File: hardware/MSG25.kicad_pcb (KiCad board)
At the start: 2 copper layers, 48 parts, among them J101 USART, J102 STLink, U105 AMS1117-5, U106 AMS1117-3.3, U202 STM32L431RCTx, U501 MCP2561-E-SN

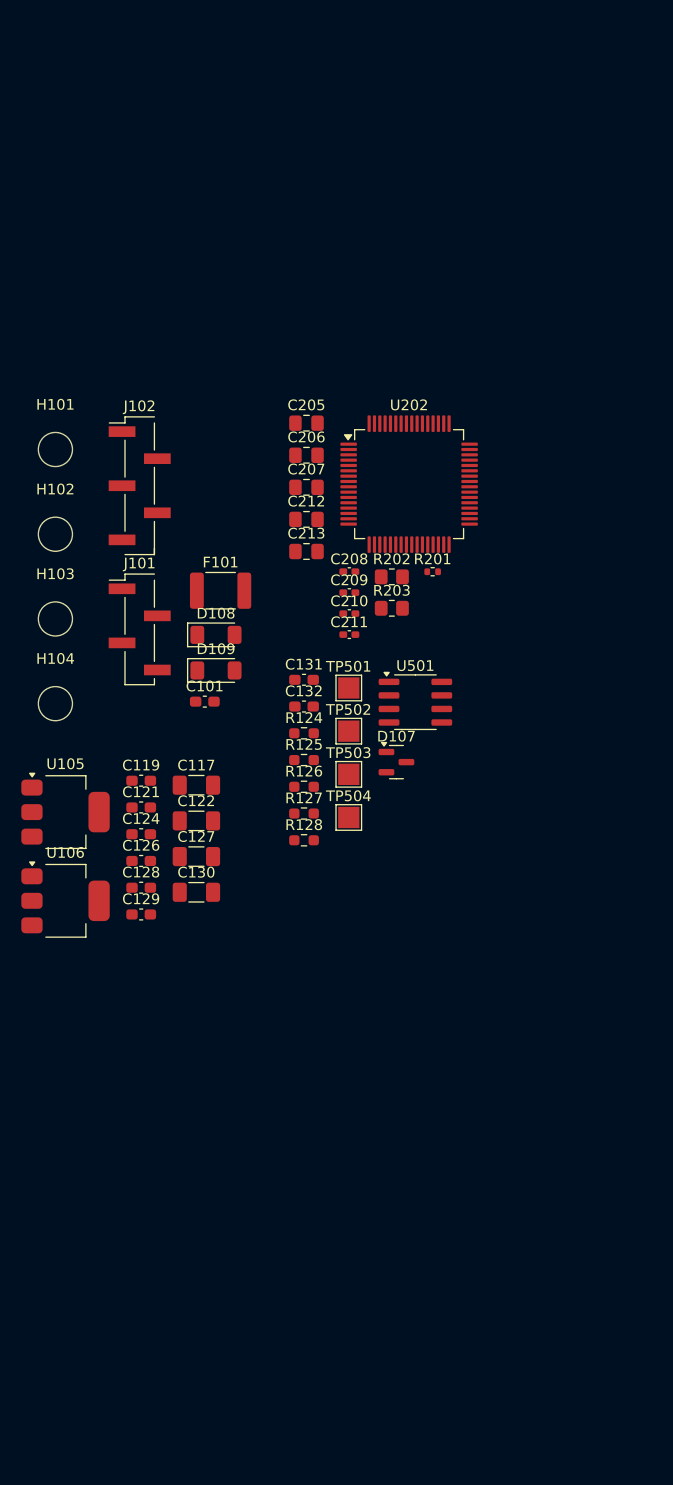
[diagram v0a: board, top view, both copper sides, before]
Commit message: Placa Finalizada para revisão
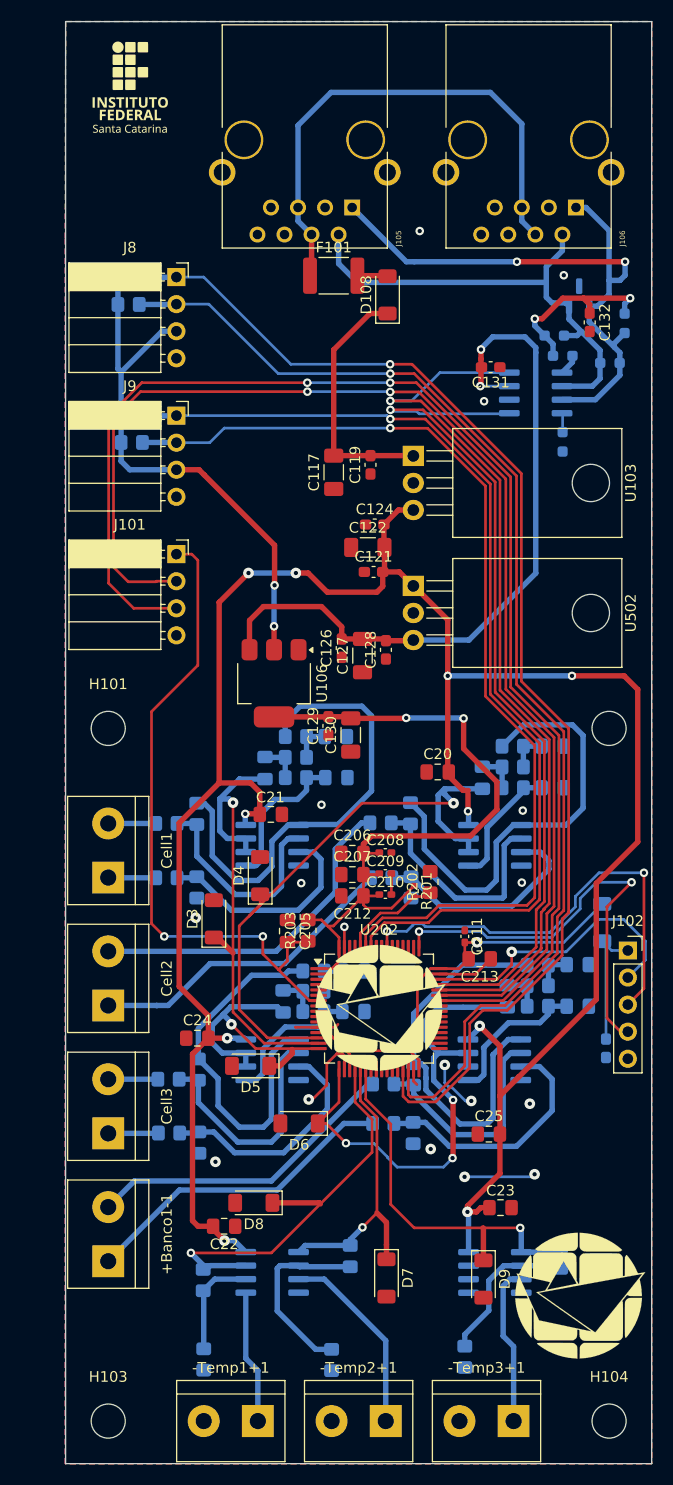
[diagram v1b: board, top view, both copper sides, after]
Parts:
- removed TP501: TxCAN, TestPoint:TestPoint_Pad_2.0x2.0mm
- removed TP502: RxCAN, TestPoint:TestPoint_Pad_2.0x2.0mm
- removed TP503: CAN_H, TestPoint:TestPoint_Pad_2.0x2.0mm
- removed TP504: CAN_L, TestPoint:TestPoint_Pad_2.0x2.0mm
- removed U105: AMS1117-5, Package_TO_SOT_SMD:SOT-223-3_TabPin2
- added +Banco1-1: Conn_01x02, TerminalBlock:TerminalBlock_bornier-2_P5.08mm, F.Cu at (115.7, 142.6)
- added -Temp1+1: Conn_01x02, TerminalBlock:TerminalBlock_bornier-2_P5.08mm, F.Cu at (129.7, 157.6)
- added -Temp2+1: Conn_01x02, TerminalBlock:TerminalBlock_bornier-2_P5.08mm, F.Cu at (141.7, 157.6)
- added -Temp3+1: Conn_01x02, TerminalBlock:TerminalBlock_bornier-2_P5.08mm, F.Cu at (153.7, 157.6)
- added C10: 100n, Capacitor_SMD:C_0805_2012Metric_Pad1.18x1.45mm_HandSolder, B.Cu at (157.4, 98.1)
- added C11: 100n, Capacitor_SMD:C_0805_2012Metric_Pad1.18x1.45mm_HandSolder, B.Cu at (138.7, 115.3)
- added C12: 100n, Capacitor_SMD:C_0805_2012Metric_Pad1.18x1.45mm_HandSolder, B.Cu at (132.1, 118.2)
- added C13: 100n, Capacitor_SMD:C_0805_2012Metric_Pad1.18x1.45mm_HandSolder, B.Cu at (138.7, 119.1)
- added C14: 100n, Capacitor_SMD:C_0805_2012Metric_Pad1.18x1.45mm_HandSolder, B.Cu at (159.8, 114.7)
- added C15: 100n, Capacitor_SMD:C_0805_2012Metric_Pad1.18x1.45mm_HandSolder, B.Cu at (153.1, 117.7)
- added C16: 100n, Capacitor_SMD:C_0805_2012Metric_Pad1.18x1.45mm_HandSolder, B.Cu at (159.8, 118.6)
- added C20: 100nF, Capacitor_SMD:C_0805_2012Metric_Pad1.18x1.45mm_HandSolder, F.Cu at (146.6, 96.6)
- added C21: 100nF, Capacitor_SMD:C_0805_2012Metric_Pad1.18x1.45mm_HandSolder, F.Cu at (131.0, 100.6)
- added C22: 100nF, Capacitor_SMD:C_0805_2012Metric_Pad1.18x1.45mm_HandSolder, F.Cu at (126.6, 139.3)
- added C23: 100nF, Capacitor_SMD:C_0805_2012Metric_Pad1.18x1.45mm_HandSolder, F.Cu at (152.5, 137.5)
- added C24: 100nF, Capacitor_SMD:C_0805_2012Metric_Pad1.18x1.45mm_HandSolder, F.Cu at (124.1, 121.6)
- added C25: 100nF, Capacitor_SMD:C_0805_2012Metric_Pad1.18x1.45mm_HandSolder, F.Cu at (151.4, 130.6)
- added C5: 100n, Capacitor_SMD:C_0805_2012Metric_Pad1.18x1.45mm_HandSolder, B.Cu at (137.1, 93.3)
- added C6: 100n, Capacitor_SMD:C_0805_2012Metric_Pad1.18x1.45mm_HandSolder, B.Cu at (157.4, 94.2)
- added C7: 100n, Capacitor_SMD:C_0805_2012Metric_Pad1.18x1.45mm_HandSolder, B.Cu at (130.4, 96.3)
- added C8: 100n, Capacitor_SMD:C_0805_2012Metric_Pad1.18x1.45mm_HandSolder, B.Cu at (150.8, 97.2)
- added C9: 100n, Capacitor_SMD:C_0805_2012Metric_Pad1.18x1.45mm_HandSolder, B.Cu at (137.1, 97.2)
- added Cell1: Conn_01x02, TerminalBlock:TerminalBlock_bornier-2_P5.08mm, F.Cu at (115.7, 106.6)
- added Cell2: Conn_01x02, TerminalBlock:TerminalBlock_bornier-2_P5.08mm, F.Cu at (115.7, 118.6)
- added Cell3: Conn_01x02, TerminalBlock:TerminalBlock_bornier-2_P5.08mm, F.Cu at (115.7, 130.6)
- added D3: 3V3, Diode_SMD:D_MiniMELF, F.Cu at (125.6, 110.4)
- added D4: 3V3, Diode_SMD:D_MiniMELF, F.Cu at (130.0, 106.4)
- added D5: 3V3, Diode_SMD:D_MiniMELF, F.Cu at (129.1, 124.2)
- added D6: 3V3, Diode_SMD:D_MiniMELF, F.Cu at (133.6, 129.6)
- added D7: 3V3, Diode_SMD:D_MiniMELF, F.Cu at (141.8, 144.1)
- added D8: 3V3, Diode_SMD:D_MiniMELF, F.Cu at (129.4, 137.1)
- added D9: 3V3, Diode_SMD:D_MiniMELF, F.Cu at (150.9, 144.2)
- added J105: RJ45, KicadZeniteSolarLibrary18:RJ45_YH59_01, F.Cu at (138.6, 43.7)
- added J106: RJ45, KicadZeniteSolarLibrary18:RJ45_YH59_01, F.Cu at (159.6, 43.7)
- added J8: I2C_1, Connector_PinSocket_2.54mm:PinSocket_1x04_P2.54mm_Horizontal, F.Cu at (122.1, 50.2)
- added J9: I2C_2, Connector_PinSocket_2.54mm:PinSocket_1x04_P2.54mm_Horizontal, F.Cu at (122.1, 63.2)
- added LOGO101: Logo_Open_Hardware_Small, Symbol:OSHW-Logo2_7.3x6mm_SilkScreen, B.Cu at (162.8, 147.3)
- added R1: 100k, Resistor_SMD:R_0805_2012Metric_Pad1.20x1.40mm_HandSolder, B.Cu at (121.2, 106.6)
- added R10: 470k, Resistor_SMD:R_0805_2012Metric_Pad1.20x1.40mm_HandSolder, B.Cu at (138.4, 142.1)
- added R11: 1k, Resistor_SMD:R_0805_2012Metric_Pad1.20x1.40mm_HandSolder, B.Cu at (124.7, 151.8)
- added R12: 15k, Resistor_SMD:R_0805_2012Metric_Pad1.20x1.40mm_HandSolder, B.Cu at (124.0, 100.6)
- added R13: 470k, Resistor_SMD:R_0805_2012Metric_Pad1.20x1.40mm_HandSolder, B.Cu at (124.6, 144.3)
- added R14: 1k, Resistor_SMD:R_0805_2012Metric_Pad1.20x1.40mm_HandSolder, B.Cu at (149.2, 151.5)
- added R15: 270k, Resistor_SMD:R_0805_2012Metric_Pad1.20x1.40mm_HandSolder, B.Cu at (158.2, 142.2)
- added R16: 100k, Resistor_SMD:R_0805_2012Metric_Pad1.20x1.40mm_HandSolder, B.Cu at (121.2, 101.5)
- added R17: 100k, Resistor_SMD:R_0805_2012Metric_Pad1.20x1.40mm_HandSolder, B.Cu at (141.3, 101.4)
- added R18: 15k, Resistor_SMD:R_0805_2012Metric_Pad1.20x1.40mm_HandSolder, B.Cu at (144.1, 100.5)
- added R19: 100k, Resistor_SMD:R_0805_2012Metric_Pad1.20x1.40mm_HandSolder, B.Cu at (121.4, 125.5)
- added R2: 15k, Resistor_SMD:R_0805_2012Metric_Pad1.20x1.40mm_HandSolder, B.Cu at (124.0, 107.5)
- added R20: 15k, Resistor_SMD:R_0805_2012Metric_Pad1.20x1.40mm_HandSolder, B.Cu at (124.2, 124.6)
- added R21: 100k, Resistor_SMD:R_0805_2012Metric_Pad1.20x1.40mm_HandSolder, B.Cu at (141.5, 125.9)
- added R22: 5k6, Resistor_SMD:R_0805_2012Metric_Pad1.20x1.40mm_HandSolder, B.Cu at (144.4, 125.0)
- added R23: 1k, Resistor_SMD:R_0805_2012Metric_Pad1.20x1.40mm_HandSolder, B.Cu at (133.3, 93.3)
- added R24: 1k, Resistor_SMD:R_0805_2012Metric_Pad1.20x1.40mm_HandSolder, B.Cu at (133.3, 95.3)
- added R25: 1k, Resistor_SMD:R_0805_2012Metric_Pad1.20x1.40mm_HandSolder, B.Cu at (133.3, 97.2)
- added R26: 1k, Resistor_SMD:R_0805_2012Metric_Pad1.20x1.40mm_HandSolder, B.Cu at (153.7, 94.2)
- added R27: 1k, Resistor_SMD:R_0805_2012Metric_Pad1.20x1.40mm_HandSolder, B.Cu at (153.7, 96.2)
- added R28: 1k, Resistor_SMD:R_0805_2012Metric_Pad1.20x1.40mm_HandSolder, B.Cu at (153.7, 98.1)
- added R29: 1k, Resistor_SMD:R_0805_2012Metric_Pad1.20x1.40mm_HandSolder, B.Cu at (135.0, 115.3)
- added R3: 100k, Resistor_SMD:R_0805_2012Metric_Pad1.20x1.40mm_HandSolder, B.Cu at (141.3, 106.6)
- added R30: 1k, Resistor_SMD:R_0805_2012Metric_Pad1.20x1.40mm_HandSolder, B.Cu at (135.0, 117.2)
- added R31: 1k, Resistor_SMD:R_0805_2012Metric_Pad1.20x1.40mm_HandSolder, B.Cu at (135.0, 119.1)
- added R32: 1k, Resistor_SMD:R_0805_2012Metric_Pad1.20x1.40mm_HandSolder, B.Cu at (156.0, 114.8)
- added R33: 1k, Resistor_SMD:R_0805_2012Metric_Pad1.20x1.40mm_HandSolder, B.Cu at (156.0, 116.7)
- added R34: 1k, Resistor_SMD:R_0805_2012Metric_Pad1.20x1.40mm_HandSolder, B.Cu at (156.0, 118.6)
- added R35: 4k7, Resistor_SMD:R_0805_2012Metric_Pad1.20x1.40mm_HandSolder, B.Cu at (117.6, 50.2)
- added R36: 4k7, Resistor_SMD:R_0805_2012Metric_Pad1.20x1.40mm_HandSolder, B.Cu at (117.6, 52.8)
- added R37: 4k7, Resistor_SMD:R_0805_2012Metric_Pad1.20x1.40mm_HandSolder, B.Cu at (117.9, 63.2)
- added R38: 4k7, Resistor_SMD:R_0805_2012Metric_Pad1.20x1.40mm_HandSolder, B.Cu at (117.9, 65.7)
- added R4: 15k, Resistor_SMD:R_0805_2012Metric_Pad1.20x1.40mm_HandSolder, B.Cu at (144.1, 107.5)
- added R5: 100k, Resistor_SMD:R_0805_2012Metric_Pad1.20x1.40mm_HandSolder, B.Cu at (121.4, 130.5)
- added R6: 15k, Resistor_SMD:R_0805_2012Metric_Pad1.20x1.40mm_HandSolder, B.Cu at (124.2, 131.4)
- added R7: 100k, Resistor_SMD:R_0805_2012Metric_Pad1.20x1.40mm_HandSolder, B.Cu at (141.5, 129.6)
- added R8: 5k6, Resistor_SMD:R_0805_2012Metric_Pad1.20x1.40mm_HandSolder, B.Cu at (144.3, 130.5)
- added R9: 1k, Resistor_SMD:R_0805_2012Metric_Pad1.20x1.40mm_HandSolder, B.Cu at (136.7, 151.8)
- added SYM101: SYM_Radioactive_Radiation_Small, KicadZeniteSolarLibrary18:symbol_logoZenite, F.Cu at (141.2, 118.7)
- added SYM102: SYM_Radioactive_Radiation_Small, KicadZeniteSolarLibrary18:symbol_logoZenite, F.Cu at (160.0, 145.8)
- added SYM103: SYM_Radioactive_Radiation_Small, KicadZeniteSolarLibrary18:symbol_naolavar, B.Cu at (160.9, 135.4)
- added SYM104: SYM_LASER_Small, KicadZeniteSolarLibrary18:synbol_logoifsc, B.Cu at (117.8, 32.4)
- added SYM105: SYM_LASER_Small, KicadZeniteSolarLibrary18:synbol_logoifsc, F.Cu at (117.8, 32.4)
- added U1: LM358, Package_SO:SOIC-8_3.9x4.9mm_P1.27mm, B.Cu at (131.1, 103.5)
- added U103: K78L15-1000R3, Package_TO_SOT_THT:TO-220-3_Horizontal_TabDown, F.Cu at (144.3, 67.0)
- added U2: LM358, Package_SO:SOIC-8_3.9x4.9mm_P1.27mm, B.Cu at (152.0, 103.5)
- added U3: LM358, Package_SO:SOIC-8_3.9x4.9mm_P1.27mm, B.Cu at (131.1, 143.6)
- added U4: LM358, Package_SO:SOIC-8_3.9x4.9mm_P1.27mm, B.Cu at (152.0, 143.6)
- added U5: LM358, Package_SO:SOIC-8_3.9x4.9mm_P1.27mm, B.Cu at (131.1, 123.7)
- added U502: LM7805, Package_TO_SOT_THT:TO-220-3_Horizontal_TabDown, F.Cu at (144.3, 79.2)
- added U6: LM358, Package_SO:SOIC-8_3.9x4.9mm_P1.27mm, B.Cu at (151.9, 123.7)
- C101, D107, D109, H102, R124, R125, R126, R127, R128, U501: moved to B.Cu
- J101: footprint Connector_PinHeader_2.54mm:PinHeader_1x04_P2.54mm_Vertical_SMD_Pin1Left -> Connector_PinSocket_2.54mm:PinSocket_1x04_P2.54mm_Horizontal
- J102: footprint Connector_PinHeader_2.54mm:PinHeader_1x05_P2.54mm_Vertical_SMD_Pin1Left -> Connector_PinSocket_2.54mm:PinSocket_1x05_P2.54mm_Vertical
- moved H104 85.0 mm to (162.7, 157.6)
- moved H103 75.4 mm to (115.7, 157.6)
- moved J102 63.2 mm to (164.5, 113.4)
- moved H102 55.1 mm to (162.7, 92.6), turned to 180 degrees
- moved R127 55.0 mm to (164.2, 54.5), turned to -90 degrees
- moved R128 52.9 mm to (157.6, 55.7), turned to 180 degrees
- moved C101 49.8 mm to (162.4, 122.6), turned to 90 degrees
- moved U202 49.3 mm to (141.1, 118.8)
- moved C205 47.7 mm to (132.5, 111.6), turned to -90 degrees
- moved R126 47.2 mm to (158.3, 57.6)
- moved R125 47.0 mm to (162.8, 58.3)
- moved D107 47.0 mm to (159.9, 52.0), turned to 90 degrees
- moved C132 44.9 mm to (160.9, 54.5), turned to -90 degrees
- moved D109 43.3 mm to (162.1, 110.8), turned to -90 degrees
- moved C213 41.5 mm to (150.6, 114.2), turned to 180 degrees
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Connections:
- net /CANBUS/5v renamed +5V
- net /POWER SUPPLY/+15V renamed +15V
- C211 pad 1: GNDA -> GND
- C213 pad 1: GNDA -> GND
- U202 pad 12: GNDA -> GND
- U202 pad 14: unconnected-(U202-PA0-Pad14) -> /ANALOG/Vcell2_a
- U202 pad 15: unconnected-(U202-PA1-Pad15) -> /ANALOG/Vcell1_a
- U202 pad 16: unconnected-(U202-PA2-Pad16) -> /ANALOG/Vcell3_a
- U202 pad 17: unconnected-(U202-PA3-Pad17) -> /ANALOG/Vbanco_a
- U202 pad 20: unconnected-(U202-PA4-Pad20) -> /ANALOG/Temp1_a
- U202 pad 21: unconnected-(U202-PA5-Pad21) -> /ANALOG/Temp2_a
- U202 pad 22: unconnected-(U202-PA6-Pad22) -> /ANALOG/Temp3_a
- U202 pad 29: unconnected-(U202-PB10-Pad29) -> /MCU/I2C_2_SCL
- U202 pad 30: unconnected-(U202-PB11-Pad30) -> /MCU/I2C_2_SDA
- U202 pad 58: unconnected-(U202-PB6-Pad58) -> /MCU/I2C_1_SCL
- U202 pad 59: unconnected-(U202-PB7-Pad59) -> /MCU/I2C_1_SDA
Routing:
- net +15V: track 0.00 -> 223.8 mm, vias 0 -> 10
- net +3V3: track 0.00 -> 163.2 mm, vias 0 -> 5
- net /MCU/USART_TX: track 0.00 -> 124.9 mm, vias 0 -> 2
- net /MCU/USART_RX: track 0.00 -> 119.9 mm, vias 0 -> 2
- net /MCU/I2C_2_SCL: track 0.00 -> 116.6 mm, vias 0 -> 1
- net /MCU/I2C_2_SDA: track 0.00 -> 113.5 mm, vias 0 -> 1
- net /MCU/I2C_1_SCL: track 0.00 -> 94.6 mm, vias 0 -> 1
- net /MCU/I2C_1_SDA: track 0.00 -> 94.1 mm, vias 0 -> 1
- net /CANBUS/CAN_RX: track 0.00 -> 83.0 mm, vias 0 -> 1
- net /CANBUS/CAN_TX: track 0.00 -> 80.4 mm, vias 0 -> 1
- net +5V: track 0.00 -> 69.1 mm, vias 0 -> 2
- net /MCU/RESET: track 0.00 -> 62.7 mm, vias 0 -> 2
- net /CANBUS CONN/CAN_H: track 0.00 -> 58.9 mm, vias 0 -> 2
- net /ANALOG/Vcell2_a: track 0.00 -> 57.1 mm, vias 0 -> 1
- net /CANBUS CONN/CAN_18V: track 0.00 -> 49.1 mm
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- added copper zone on B.Cu, net GND
- added copper zone on F.Cu, net GND
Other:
- board outline added: 55 x 135.3 mm
